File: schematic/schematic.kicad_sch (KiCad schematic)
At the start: 29 parts, among them J1 Screw_Terminal_01x16, J2 Screw_Terminal_01x06, J6 Screw_Terminal_01x06, K2 External relay for dust colle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, K5 Pressure sensor relay, M1 Dust collector motor, M2 16-channel multiplexer, Q1 IRF520N, U1 ESP32-WROOM-32, U2 DS18B20, U4 Ultrasonic range sensor, U5 Scale Module

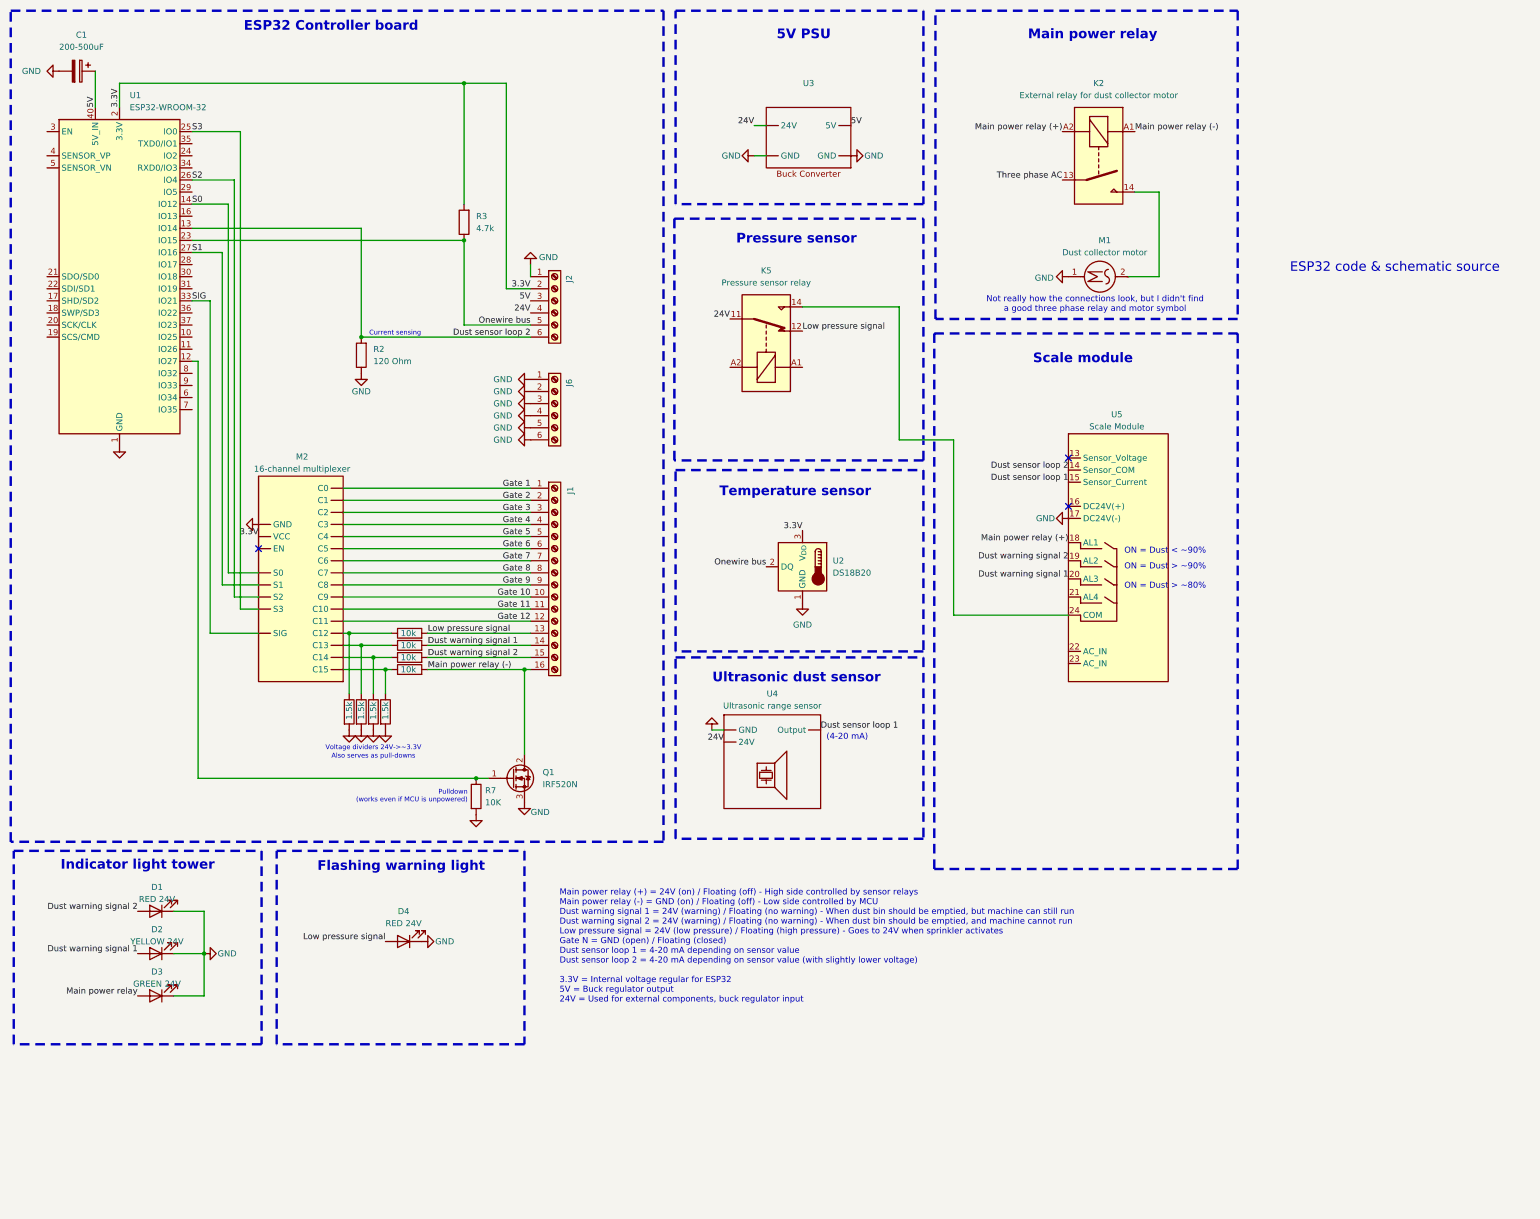
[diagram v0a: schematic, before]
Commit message: Update schematic.
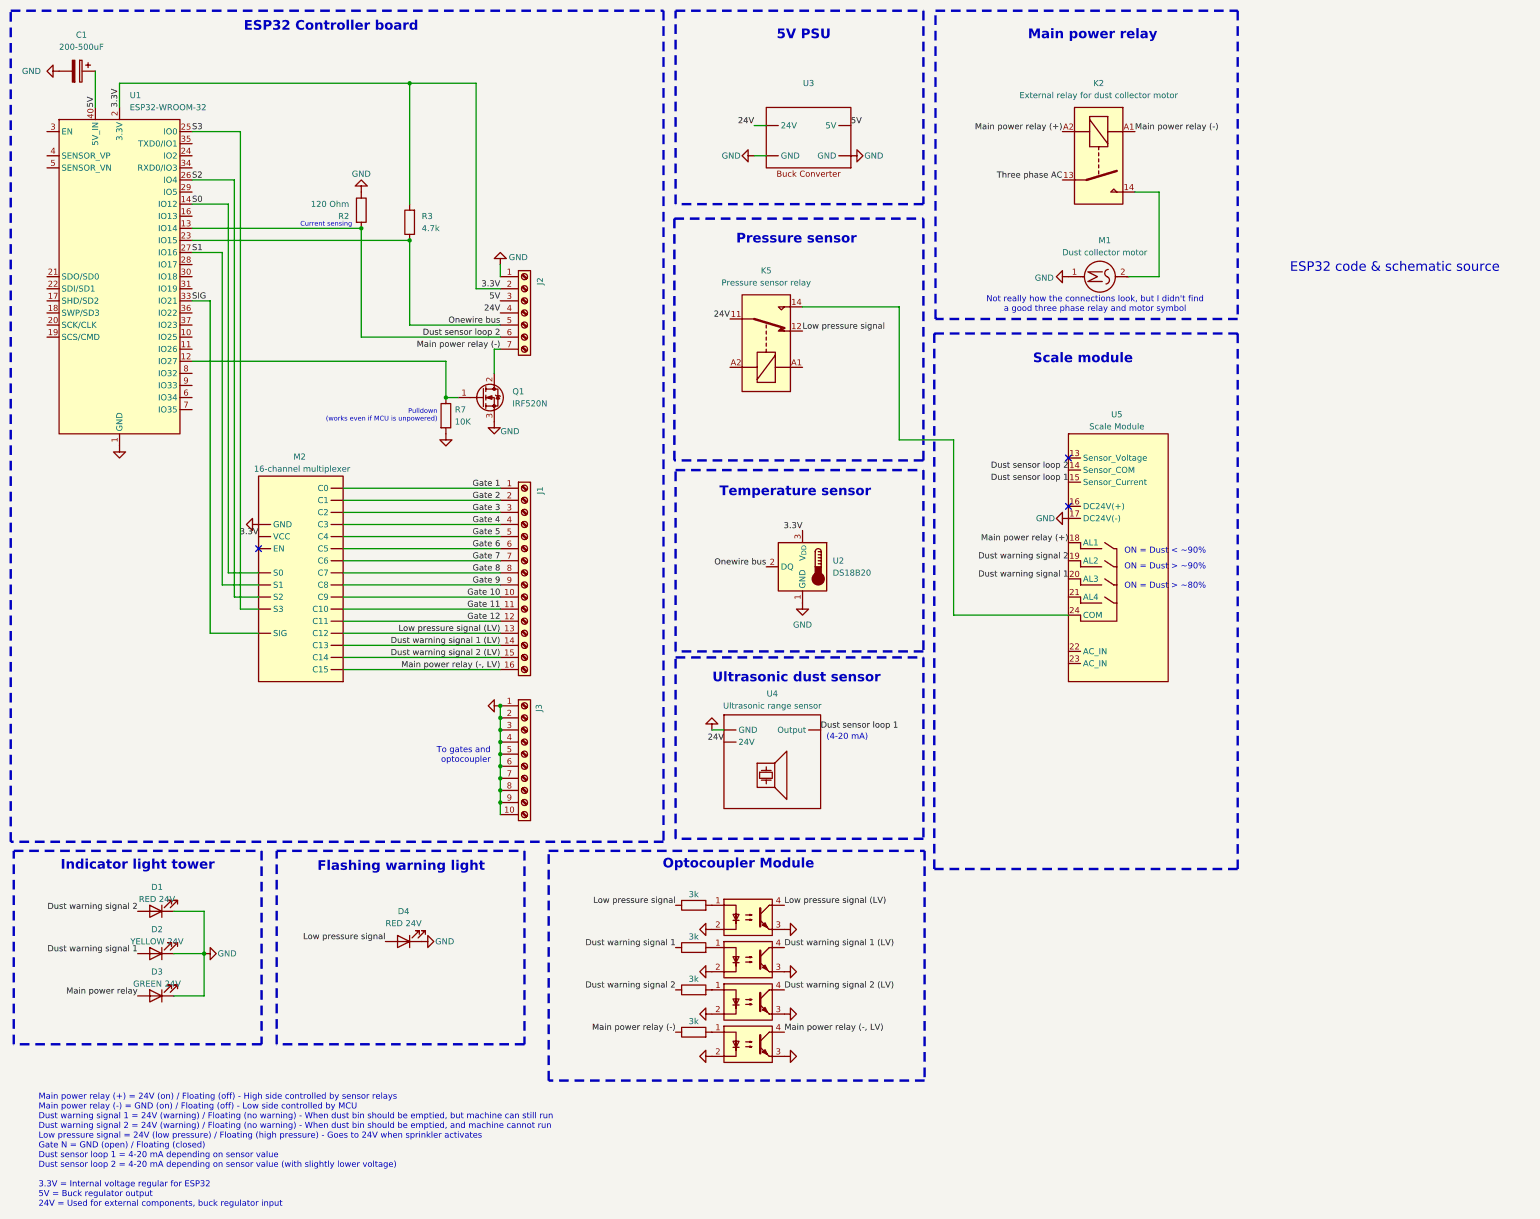
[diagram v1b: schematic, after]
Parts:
- removed J2, J6: Screw_Terminal_01x06, symbol Connector:Screw_Terminal_01x06
- removed R11, R12, R13, R14: 1.5k, symbol Device:R
- removed R8, R9: 10k, symbol Device:R
- added J2: Screw_Terminal_01x07, symbol Connector:Screw_Terminal_01x07
- added J3: Screw_Terminal_01x10, symbol Connector:Screw_Terminal_01x10
- added R5, R6: 3k, symbol Device:R
- added U6, U7, U8, U9: Optocoupler_DC_PhotoNPN_AKEC, symbol Isolator:Optocoupler_DC_PhotoNPN_AKEC
- R1, R4: value 10k -> 3k
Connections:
- net 24V: now also J2.4 (Pin_4)
- net 3.3V: now also J2.2 (Pin_2)
- net 5V: now also J2.3 (Pin_3)
- net Dust sensor loop 2: now also J2.6 (Pin_6)
- net Dust warning signal 1: now also R4.1; no longer J1.14 (Pin_14), R1.2
- net Dust warning signal 2: now also R5.1; no longer J1.15 (Pin_15)
- net GND: now also J2.1 (Pin_1), J3.1 (Pin_1), J3.10 (Pin_10), J3.2 (Pin_2), J3.3 (Pin_3), J3.4 (Pin_4), J3.5 (Pin_5), J3.6 (Pin_6), J3.7 (Pin_7), J3.8 (Pin_8), J3.9 (Pin_9), U6.2, U6.3, U7.2, U7.3, U8.2, U8.3, U9.2, U9.3
- net Low pressure signal: now also R1.1; no longer J1.13 (Pin_13)
- net Main power relay (-): now also J2.7 (Pin_7), R6.1; no longer J1.16 (Pin_16), R4.2
- net Onewire bus: now also J2.5 (Pin_5)
- new net: R4.2, U7.1
- new net: R6.2, U9.1
- new net: R5.2, U8.1
- new net: R1.2, U6.1
- new net Dust warning signal 1 (LV): J1.14 (Pin_14), M2. (GND), U7.4
- new net Dust warning signal 2 (LV): J1.15 (Pin_15), M2. (GND), U8.4
- new net Low pressure signal (LV): J1.13 (Pin_13), M2. (GND), U6.4
- new net Main power relay (-, LV): J1.16 (Pin_16), M2. (GND), U9.4
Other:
- note added: "Optocoupler Module"
- note added: "To gates and optocoupler"
- note removed: "Also serves as pull-downs"
- note removed: "Voltage dividers 24V->~3.3V"
- moved on the sheet: J1, Q1, R2, R3, R7
